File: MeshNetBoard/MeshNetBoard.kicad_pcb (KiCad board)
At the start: 4 copper layers, 65 x 30 mm, 41 parts, among them J2 Conn_01x02, J3 Micro_SD_Card_Det_Hirose_DM3AT, Q1 Q_PMOS_GSD, SW1 SW_Push, SW2 SW_SPST, U1 XIAO-ESP32-S3-DIP, U2 TPS631000DRLR, U4 MAX9031AU, U5 MCP73831-2-OT

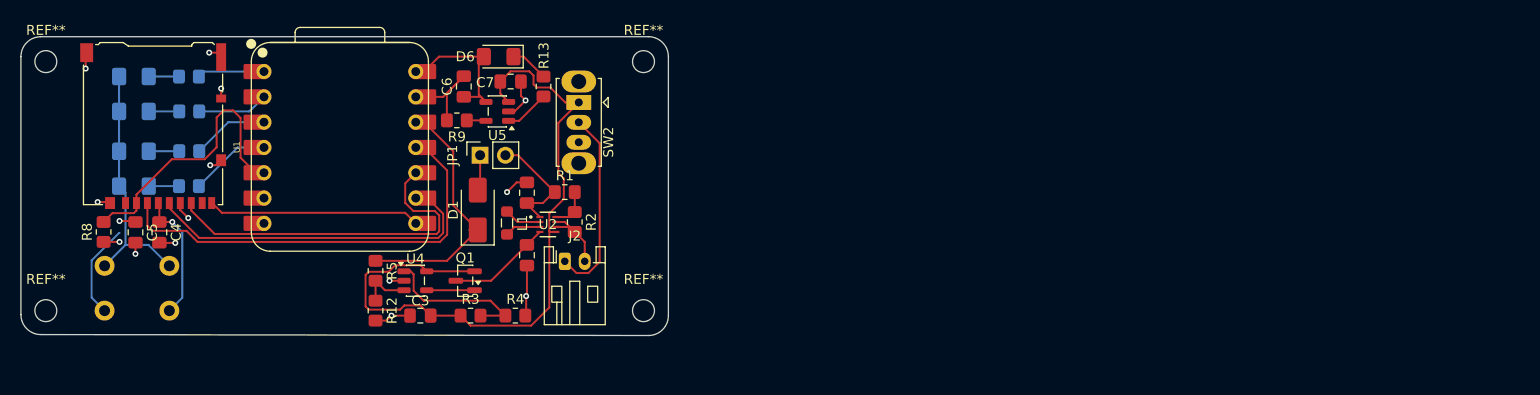
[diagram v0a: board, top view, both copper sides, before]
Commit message: maybe doen
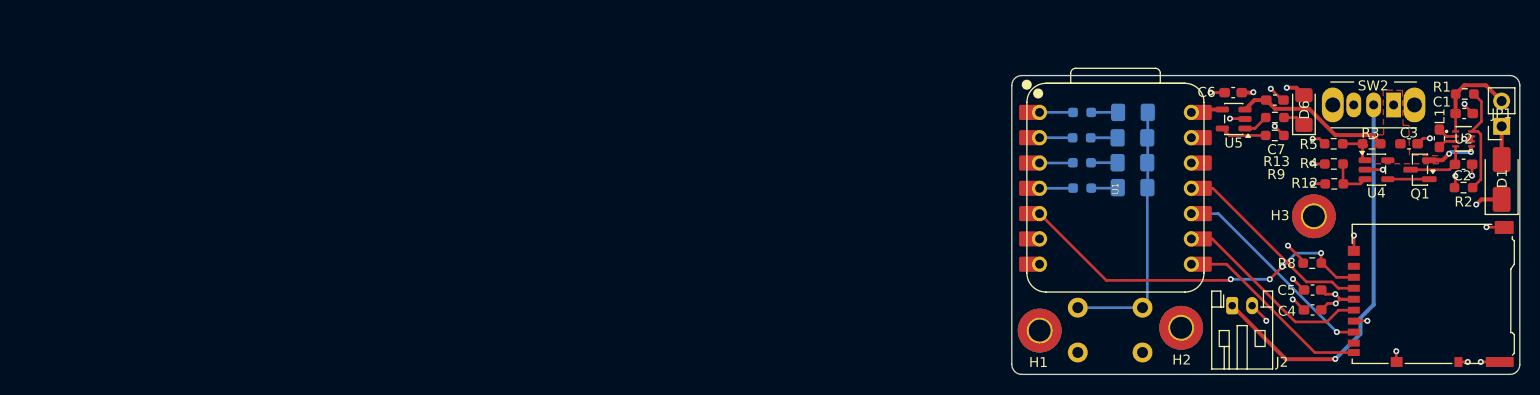
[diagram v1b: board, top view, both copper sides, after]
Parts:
- removed REF** (x4): MountingHole_2.2mm_M2, MountingHole:MountingHole_2.2mm_M2
- added H1: MountingHole_Pad, MountingHole:MountingHole_2.2mm_M2_Pad_TopBottom, F.Cu at (154.5, 51.0)
- added H2: MountingHole_Pad, MountingHole:MountingHole_2.2mm_M2_Pad_TopBottom, F.Cu at (168.7, 50.7)
- added H3: MountingHole_Pad, MountingHole:MountingHole_2.2mm_M2_Pad_TopBottom, F.Cu at (182.0, 39.5)
- C1, C2, C3, C4, C5, C6, C7: footprint Capacitor_SMD:C_0805_2012Metric_Pad1.18x1.45mm_HandSolder -> Capacitor_SMD:C_0603_1608Metric_Pad1.08x0.95mm_HandSolder
- L1: footprint Inductor_SMD:L_0805_2012Metric_Pad1.05x1.20mm_HandSolder -> Inductor_SMD:L_0603_1608Metric_Pad1.05x0.95mm_HandSolder
- R1, R10, R11, R12, R13, R2, R3, R4, R5, R6, R7, R8, R9: footprint Resistor_SMD:R_0805_2012Metric_Pad1.20x1.40mm_HandSolder -> Resistor_SMD:R_0603_1608Metric_Pad0.98x0.95mm_HandSolder
- SW2: footprint Button_Switch_THT:SW_Slide_SPDT_Straight_CK_OS102011MS2Q -> Button_Switch_THT:SW_Slide_SPDT_Angled_CK_OS102011MA1Q
- moved J3 129.4 mm to (193.7, 47.3), turned to 90 degrees
- moved R8 121.4 mm to (181.8, 44.2), turned to 0 degrees
- moved C5 118.3 mm to (181.9, 46.9), turned to 180 degrees
- moved C4 116.0 mm to (181.9, 48.9), turned to 180 degrees
- moved D1 102.8 mm to (200.8, 35.8)
- moved JP1 102.6 mm to (200.8, 30.5), turned to 180 degrees
- moved C3 100.7 mm to (191.6, 32.2), turned to 180 degrees
- moved D2 100.4 mm to (163.8, 29.1), turned to 0 degrees
- moved D3 100.3 mm to (163.8, 31.6), turned to 0 degrees
- moved D5 100.3 mm to (163.8, 36.6), turned to 0 degrees
- moved D4 100.3 mm to (163.8, 34.1), turned to 0 degrees
- moved SW1 97.8 mm to (164.8, 48.7)
- moved U4 97.1 mm to (188.3, 34.9)
- moved R12 97.1 mm to (184.1, 36.3), turned to 180 degrees
- moved R5 96.8 mm to (184.0, 34.3), turned to 0 degrees
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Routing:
- net +BATT: track 70.6 -> 21.6 mm, vias 0 -> 2
- net 3v3: track 51.5 -> 13.8 mm, vias 3 -> 5
- net MOSI: track 43.1 -> 19.6 mm
- net Net-(J2-Pin_1): track 19.3 -> 39.7 mm, vias 0 -> 1
- net GND: track 46.6 -> 31.7 mm, vias 13 -> 21
- net SCK: track 34.0 -> 19.4 mm
- net MISO: track 35.8 -> 21.2 mm, vias 0 -> 1
- net Net-(U4-+): track 15.5 -> 4.26 mm
- net SD_DATA: track 27.5 -> 37.0 mm, vias 0 -> 4
- net 5v: track 14.1 -> 6.27 mm, vias 0 -> 2
- net Net-(U2-FB): track 4.11 -> 11.2 mm
- net LED4: track 8.14 -> 3.37 mm
- net Net-(Q1-D): track 11.2 -> 6.57 mm
- net LED3: track 7.71 -> 3.36 mm
- net LED2: track 7.10 -> 3.32 mm
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- added copper zone on F.Cu, net +BATT
- added copper zone on In2.Cu, net 5v
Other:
- board size 65 x 30 mm -> 51 x 30 mm
